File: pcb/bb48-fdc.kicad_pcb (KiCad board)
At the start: 2 copper layers, 71.1 x 61 mm, 10 parts, among them J1 FDD 34-pin host, J2 P2000T_EXPANSION_PORT, U1 74LS06, U2 74LS06, U3 74LVC14

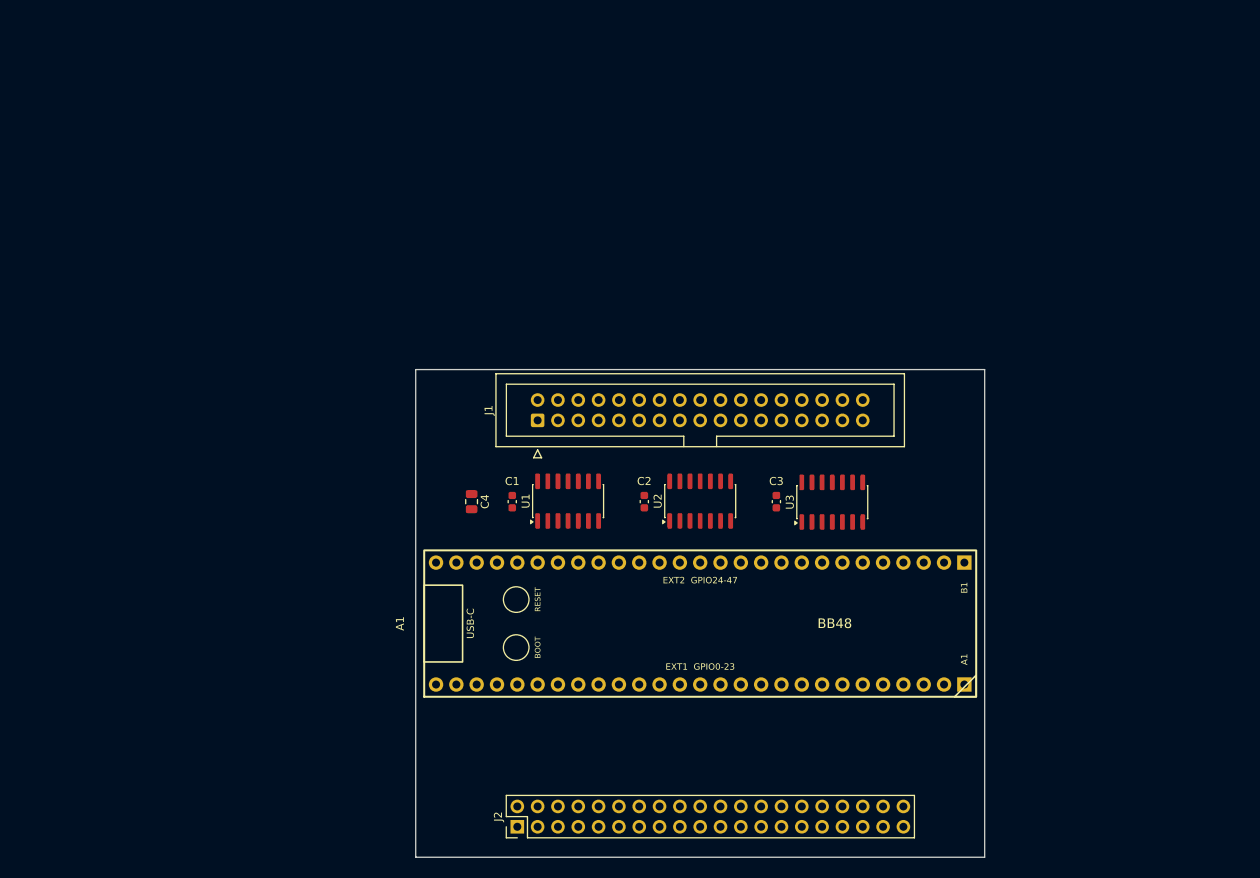
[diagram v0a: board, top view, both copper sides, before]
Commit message: Revising design
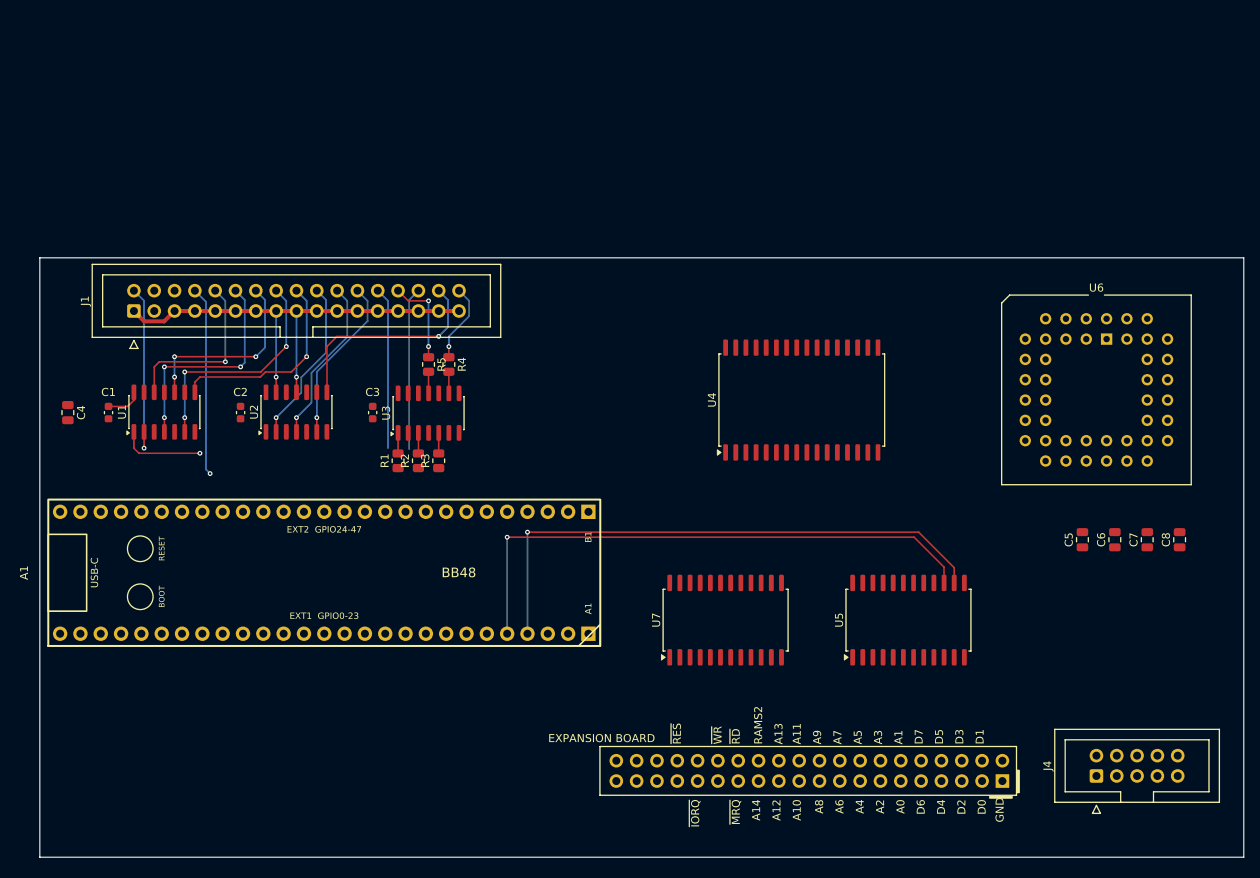
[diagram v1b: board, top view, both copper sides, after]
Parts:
- added C5: 0.1uF, Capacitor_SMD:C_0805_2012Metric, F.Cu at (106.2, 83.5)
- added C6: 0.1uF, Capacitor_SMD:C_0805_2012Metric, F.Cu at (110.2, 83.5)
- added C7: 0.1uF, Capacitor_SMD:C_0805_2012Metric, F.Cu at (114.3, 83.5)
- added C8: 0.1uF, Capacitor_SMD:C_0805_2012Metric, F.Cu at (118.3, 83.5)
- added J4: Atmel-JTAG-10, Connector_IDC:IDC-Header_2x05_P2.54mm_Vertical, F.Cu at (108.0, 113.0)
- added R1: 1k, Resistor_SMD:R_0805_2012Metric, F.Cu at (20.7, 73.6)
- added R2: 1k, Resistor_SMD:R_0805_2012Metric, F.Cu at (23.2, 73.6)
- added R3: 1k, Resistor_SMD:R_0805_2012Metric, F.Cu at (25.7, 73.6)
- added R4: 1k, Resistor_SMD:R_0805_2012Metric, F.Cu at (27.0, 61.6)
- added R5: 1k, Resistor_SMD:R_0805_2012Metric, F.Cu at (24.5, 61.6)
- added U4: CY62128Exx-xxS, Package_SO:SOP-32_11.305x20.495mm_P1.27mm, F.Cu at (71.1, 66.0)
- added U5: SN74LVC8T245, Package_SO:SOIC-24W_7.5x15.4mm_P1.27mm, F.Cu at (84.5, 93.5)
- added U6: ATF1502AS, Package_LCC:PLCC-44_THT-Socket, F.Cu at (109.2, 58.4)
- added U7: SN74LVC8T245, Package_SO:SOIC-24W_7.5x15.4mm_P1.27mm, F.Cu at (61.6, 93.5)
- C1, C2, C3: value 100n -> 0.1uF
- J2: moved to B.Cu
- moved J2 60.9 mm to (96.2, 113.7)
- moved J1 52.3 mm to (-12.4, 54.9)
- moved U3 51.7 mm to (24.5, 67.7)
- moved C2 51.7 mm to (0.97, 67.6)
- moved C4 51.7 mm to (-20.6, 67.6)
- moved U2 51.7 mm to (7.96, 67.5)
- moved C1 51.7 mm to (-15.5, 67.6)
- moved U1 51.7 mm to (-8.55, 67.5)
- moved C3 51.7 mm to (17.5, 67.6)
- moved A1 47.4 mm to (11.4, 87.6)
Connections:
- A1 pad A10: unconnected-(A1-GPIO6/UEXT_SCK-PadA10) -> MCU_D1
- A1 pad A11: unconnected-(A1-GPIO7/UEXT_MOSI-PadA11) -> MCU_D0
- A1 pad A16: unconnected-(A1-GPIO12-PadA16) -> ~{MCU_DEW}
- A1 pad A17: unconnected-(A1-GPIO13-PadA17) -> ~{MCU_FDC_CS}
- A1 pad A18: unconnected-(A1-GPIO14-PadA18) -> MCU_PHI
- A1 pad A19: unconnected-(A1-GPIO15-PadA19) -> ~{MCU_RES}
- A1 pad A20: unconnected-(A1-GPIO16-PadA20) -> ~{MCU_WR}
- A1 pad A21: unconnected-(A1-GPIO17-PadA21) -> ~{MCU_RD}
- A1 pad A22: unconnected-(A1-GPIO18-PadA22) -> MCU_A1
- A1 pad A23: unconnected-(A1-GPIO19-PadA23) -> MCU_A0
- A1 pad A24: unconnected-(A1-GPIO20-PadA24) -> MCU_READY
- A1 pad A4: unconnected-(A1-GPIO0/UEXT_TX-PadA4) -> MCU_D7
- A1 pad A5: unconnected-(A1-GPIO1/UEXT_RX-PadA5) -> MCU_D6
- A1 pad A6: unconnected-(A1-GPIO2/SDA(UEXT,QWIIC)-PadA6) -> MCU_D5
- A1 pad A7: unconnected-(A1-GPIO3/SCL(UEXT,QWIIC)-PadA7) -> MCU_D4
- A1 pad A8: unconnected-(A1-GPIO4/UEXT_MISO-PadA8) -> MCU_D3
- A1 pad A9: unconnected-(A1-GPIO5/UEXT_CS-PadA9) -> MCU_D2
- A1 pad B21: unconnected-(A1-GPIO41/ADC1-PadB21) -> INT_ASSERT
- J2 pad 1: unconnected-(J2-GND-Pad1) -> GND
- J2 pad 10: unconnected-(J2-D7-Pad10) -> D7
- J2 pad 11: unconnected-(J2-A0-Pad11) -> A0
- J2 pad 12: unconnected-(J2-A1-Pad12) -> A1
- J2 pad 13: unconnected-(J2-A2-Pad13) -> A2
- J2 pad 14: unconnected-(J2-A3-Pad14) -> A3
- J2 pad 15: unconnected-(J2-A4-Pad15) -> A4
- J2 pad 16: unconnected-(J2-A5-Pad16) -> A5
- J2 pad 17: unconnected-(J2-A6-Pad17) -> A6
- J2 pad 18: unconnected-(J2-A7-Pad18) -> A7
- J2 pad 19: unconnected-(J2-A8-Pad19) -> A8
- J2 pad 20: unconnected-(J2-A9-Pad20) -> A9
- J2 pad 21: unconnected-(J2-A10-Pad21) -> A10
- J2 pad 22: unconnected-(J2-A11-Pad22) -> A11
- J2 pad 23: unconnected-(J2-A12-Pad23) -> A12
- J2 pad 24: unconnected-(J2-A13-Pad24) -> A13
- J2 pad 25: unconnected-(J2-A14-Pad25) -> A14
- J2 pad 26: unconnected-(J2-RAMS2-Pad26) -> RAMS2
- J2 pad 27: unconnected-(J2-~{MRQ}-Pad27) -> ~{MRQ}
- J2 pad 28: unconnected-(J2-~{RD}-Pad28) -> ~{RD}
- J2 pad 29: unconnected-(J2-~{INT}-Pad29) -> ~{INT}
- J2 pad 3: unconnected-(J2-D0-Pad3) -> D0
- J2 pad 30: unconnected-(J2-~{WR}-Pad30) -> ~{WR}
- J2 pad 31: unconnected-(J2-~{IORQ}-Pad31) -> ~{IORQ}
- J2 pad 32: unconnected-(J2-~{WAIT}-Pad32) -> ~{WAIT}
- J2 pad 33: unconnected-(J2-~{M1}-Pad33) -> ~{M1}
- J2 pad 34: unconnected-(J2-~{RES}-Pad34) -> ~{RES}
- J2 pad 36: unconnected-(J2-~{RFSH}-Pad36) -> ~{RFSH}
- J2 pad 37: unconnected-(J2-~{DEW/R2425}-Pad37) -> ~{DEW}
- J2 pad 38: unconnected-(J2-PHI-Pad38) -> PHI
- J2 pad 39: unconnected-(J2-PHI2-Pad39) -> PHI2
- J2 pad 4: unconnected-(J2-D1-Pad4) -> D1
- J2 pad 40: unconnected-(J2-T4M-Pad40) -> T4M
- J2 pad 5: unconnected-(J2-D2-Pad5) -> D2
- J2 pad 6: unconnected-(J2-D3-Pad6) -> D3
- J2 pad 7: unconnected-(J2-D4-Pad7) -> D4
- J2 pad 8: unconnected-(J2-D5-Pad8) -> D5
- J2 pad 9: unconnected-(J2-D6-Pad9) -> D6
- U2 pad 10: unconnected-(U2-Pad10) -> ~{INT}
- U2 pad 11: GND -> INT_ASSERT
- U2 pad 12: unconnected-(U2-Pad12) -> ~{WAIT}
- U2 pad 13: GND -> WAIT_ASSERT
- U3 pad 1: ~{FDD_INDEX} -> Net-(R1-Pad2)
- U3 pad 11: ~{FDD_WPT} -> Net-(R5-Pad2)
- U3 pad 3: ~{FDD_TRK0} -> Net-(R2-Pad2)
- U3 pad 5: ~{FDD_RDATA} -> Net-(R3-Pad2)
- U3 pad 9: ~{FDD_DSKCHG} -> Net-(R4-Pad2)
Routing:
- net MCU_D6: track 0.00 -> 70.2 mm, vias 0 -> 1
- net MCU_D7: track 0.00 -> 69.8 mm, vias 0 -> 1
- net GND: track 0.00 -> 62.0 mm, vias 0 -> 2
- net ~{FDD_MOTEB}: track 0.00 -> 29.0 mm, vias 0 -> 3
- net ~{FDD_DRVSB}: track 0.00 -> 27.9 mm, vias 0 -> 3
- net ~{FDD_SIDE1}: track 0.00 -> 26.9 mm, vias 0 -> 1
- net ~{FDD_DIR}: track 0.00 -> 25.3 mm, vias 0 -> 1
- net ~{FDD_DRVSA}: track 0.00 -> 23.8 mm, vias 0 -> 3
- net ~{FDD_INDEX}: track 0.00 -> 23.6 mm, vias 0 -> 1
- net ~{FDD_DENSEL}: track 0.00 -> 22.2 mm, vias 0 -> 1
- net ~{FDD_MOTEA}: track 0.00 -> 21.7 mm, vias 0 -> 1
- net ~{FDD_WGATE}: track 0.00 -> 20.8 mm, vias 0 -> 1
- net ~{FDD_WDATA}: track 0.00 -> 20.8 mm, vias 0 -> 1
- net ~{FDD_STEP}: track 0.00 -> 20.7 mm, vias 0 -> 1
- net ~{FDD_RDATA}: track 0.00 -> 20.3 mm
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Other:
- board size 71.1 x 61 mm -> 150.5 x 74.9 mm
- board text added: "A0"
- board text added: "A1"
- board text added: "A10"
- board text added: "A11"
- board text added: "A12"
- board text added: "A13"
- board text added: "A14"
- board text added: "A2"
- board text added: "A3"
- board text added: "A4"
- board text added: "A5"
- board text added: "A6"
- board text added: "A7"
- board text added: "A8"
- board text added: "A9"
- board text added: "D0"
- board text added: "D1"
- board text added: "D2"
- board text added: "D3"
- board text added: "D4"
- board text added: "D5"
- board text added: "D6"
- board text added: "D7"
- board text added: "EXPANSION BOARD"
- board text added: "GND"
- board text added: "RAMS2"
- board text added: "~{IORQ}"
- board text added: "~{MRQ}"
- board text added: "~{RD}"
- board text added: "~{RES}"
- board text added: "~{WR}"

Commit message: Cleaning up schematic
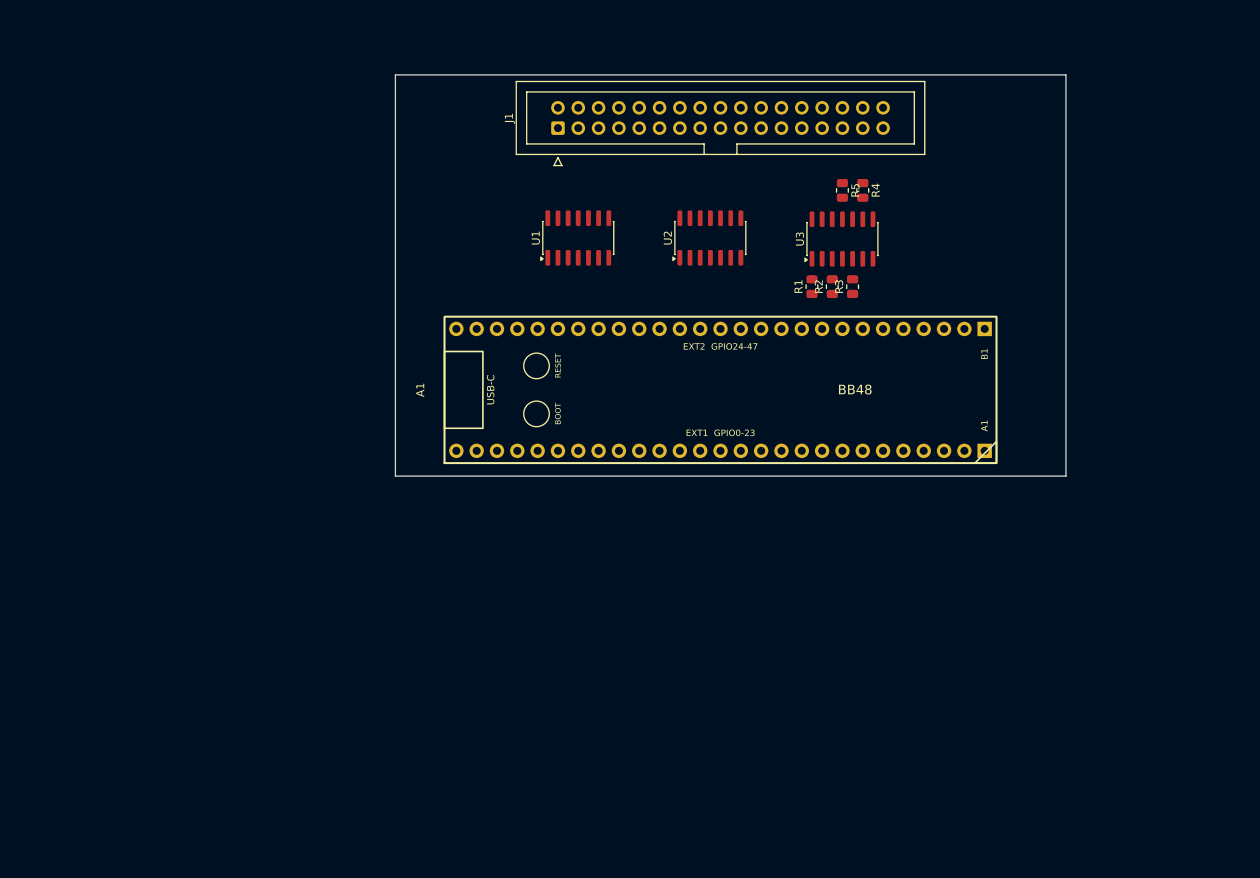
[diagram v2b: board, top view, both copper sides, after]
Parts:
- removed C1, C2, C3: 0.1uF, Capacitor_SMD:C_0603_1608Metric
- removed C4: 4.7u, Capacitor_SMD:C_0805_2012Metric
- removed C5, C6, C7, C8: 0.1uF, Capacitor_SMD:C_0805_2012Metric
- removed J2: P2000T_EXPANSION_PORT, Connector_PinHeader_2.54mm:PinHeader_2x20_P2.54mm_Vertical
- removed J4: Atmel-JTAG-10, Connector_IDC:IDC-Header_2x05_P2.54mm_Vertical
- removed U4: CY62128Exx-xxS, Package_SO:SOP-32_11.305x20.495mm_P1.27mm
- removed U5, U7: SN74LVC8T245, Package_SO:SOIC-24W_7.5x15.4mm_P1.27mm
- removed U6: ATF1502AS, Package_LCC:PLCC-44_THT-Socket
- moved J1 57.7 mm to (40.6, 32.0)
- moved R2 56.1 mm to (74.9, 51.9)
- moved R1 56.1 mm to (72.4, 51.9)
- moved R3 56.1 mm to (77.5, 51.9)
- moved R4 56.1 mm to (78.7, 39.8)
- moved R5 56.1 mm to (76.2, 39.8)
- moved U1 56.1 mm to (43.2, 45.8)
- moved U2 56.1 mm to (59.7, 45.8)
- moved U3 56.1 mm to (76.2, 45.9)
- moved A1 54.6 mm to (61.0, 64.8)
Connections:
- A1 pad A10: MCU_D1 -> unconnected-(A1-GPIO6/UEXT_SCK-PadA10)
- A1 pad A11: MCU_D0 -> unconnected-(A1-GPIO7/UEXT_MOSI-PadA11)
- A1 pad A16: ~{MCU_DEW} -> unconnected-(A1-GPIO12-PadA16)
- A1 pad A17: ~{MCU_FDC_CS} -> unconnected-(A1-GPIO13-PadA17)
- A1 pad A18: MCU_PHI -> unconnected-(A1-GPIO14-PadA18)
- A1 pad A19: ~{MCU_RES} -> unconnected-(A1-GPIO15-PadA19)
- A1 pad A20: ~{MCU_WR} -> unconnected-(A1-GPIO16-PadA20)
- A1 pad A21: ~{MCU_RD} -> unconnected-(A1-GPIO17-PadA21)
- A1 pad A22: MCU_A1 -> unconnected-(A1-GPIO18-PadA22)
- A1 pad A23: MCU_A0 -> unconnected-(A1-GPIO19-PadA23)
- A1 pad A24: MCU_READY -> unconnected-(A1-GPIO20-PadA24)
- A1 pad A4: MCU_D7 -> unconnected-(A1-GPIO0/UEXT_TX-PadA4)
- A1 pad A5: MCU_D6 -> unconnected-(A1-GPIO1/UEXT_RX-PadA5)
- A1 pad A6: MCU_D5 -> unconnected-(A1-GPIO2/SDA(UEXT,QWIIC)-PadA6)
- A1 pad A7: MCU_D4 -> unconnected-(A1-GPIO3/SCL(UEXT,QWIIC)-PadA7)
- A1 pad A8: MCU_D3 -> unconnected-(A1-GPIO4/UEXT_MISO-PadA8)
- A1 pad A9: MCU_D2 -> unconnected-(A1-GPIO5/UEXT_CS-PadA9)
- A1 pad B21: INT_ASSERT -> unconnected-(A1-GPIO41/ADC1-PadB21)
- J1 pad 3: unconnected-(J1-KEY-Pad3) -> GND
- U2 pad 10: ~{INT} -> unconnected-(U2-Pad10)
- U2 pad 11: INT_ASSERT -> GND
- U2 pad 12: ~{WAIT} -> unconnected-(U2-Pad12)
- U2 pad 13: WAIT_ASSERT -> GND
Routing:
- net MCU_D6: track 70.2 -> 0.00 mm, vias 1 -> 0
- net MCU_D7: track 69.8 -> 0.00 mm, vias 1 -> 0
- net GND: track 62.0 -> 0.00 mm, vias 2 -> 0
- net ~{FDD_MOTEB}: track 29.0 -> 0.00 mm, vias 3 -> 0
- net ~{FDD_DRVSB}: track 27.9 -> 0.00 mm, vias 3 -> 0
- net ~{FDD_SIDE1}: track 26.9 -> 0.00 mm, vias 1 -> 0
- net ~{FDD_DIR}: track 25.3 -> 0.00 mm, vias 1 -> 0
- net ~{FDD_DRVSA}: track 23.8 -> 0.00 mm, vias 3 -> 0
- net ~{FDD_INDEX}: track 23.6 -> 0.00 mm, vias 1 -> 0
- net ~{FDD_DENSEL}: track 22.2 -> 0.00 mm, vias 1 -> 0
- net ~{FDD_MOTEA}: track 21.7 -> 0.00 mm, vias 1 -> 0
- net ~{FDD_WGATE}: track 20.8 -> 0.00 mm, vias 1 -> 0
- net ~{FDD_WDATA}: track 20.8 -> 0.00 mm, vias 1 -> 0
- net ~{FDD_STEP}: track 20.7 -> 0.00 mm, vias 1 -> 0
- net ~{FDD_RDATA}: track 20.3 -> 0.00 mm
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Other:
- board size 150.5 x 74.9 mm -> 83.8 x 50.1 mm
- board text removed: "A0"
- board text removed: "A1"
- board text removed: "A10"
- board text removed: "A11"
- board text removed: "A12"
- board text removed: "A13"
- board text removed: "A14"
- board text removed: "A2"
- board text removed: "A3"
- board text removed: "A4"
- board text removed: "A5"
- board text removed: "A6"
- board text removed: "A7"
- board text removed: "A8"
- board text removed: "A9"
- board text removed: "D0"
- board text removed: "D1"
- board text removed: "D2"
- board text removed: "D3"
- board text removed: "D4"
- board text removed: "D5"
- board text removed: "D6"
- board text removed: "D7"
- board text removed: "EXPANSION BOARD"
- board text removed: "GND"
- board text removed: "RAMS2"
- board text removed: "~{IORQ}"
- board text removed: "~{MRQ}"
- board text removed: "~{RD}"
- board text removed: "~{RES}"
- board text removed: "~{WR}"
